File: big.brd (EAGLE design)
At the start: 77.6 x 137.2 mm, 137 parts, among them IC1 ULN2003AD, IC2 TB6612FNG, IC3 FXAS21002C, IC4 LD117ADT50TR, IC5 MCP1825, IC6 FXAS21002C, Q1 TEFT4300, Q2 TEFT4300, Q3 TEFT4300, Q4 TEFT4300, Q5 TEFT4300, Q6 TEFT4300, Q7 8MHz

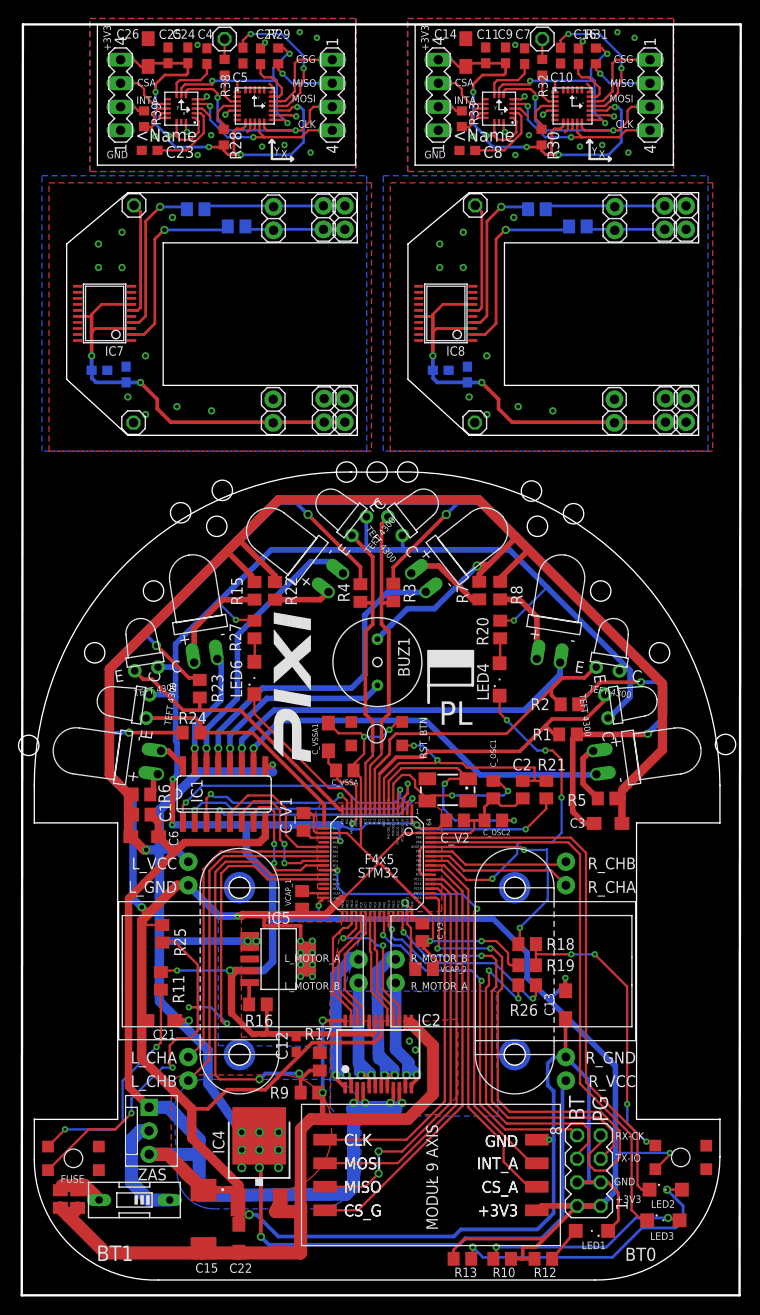
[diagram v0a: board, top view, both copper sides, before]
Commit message: schamat kodu z CubeMX
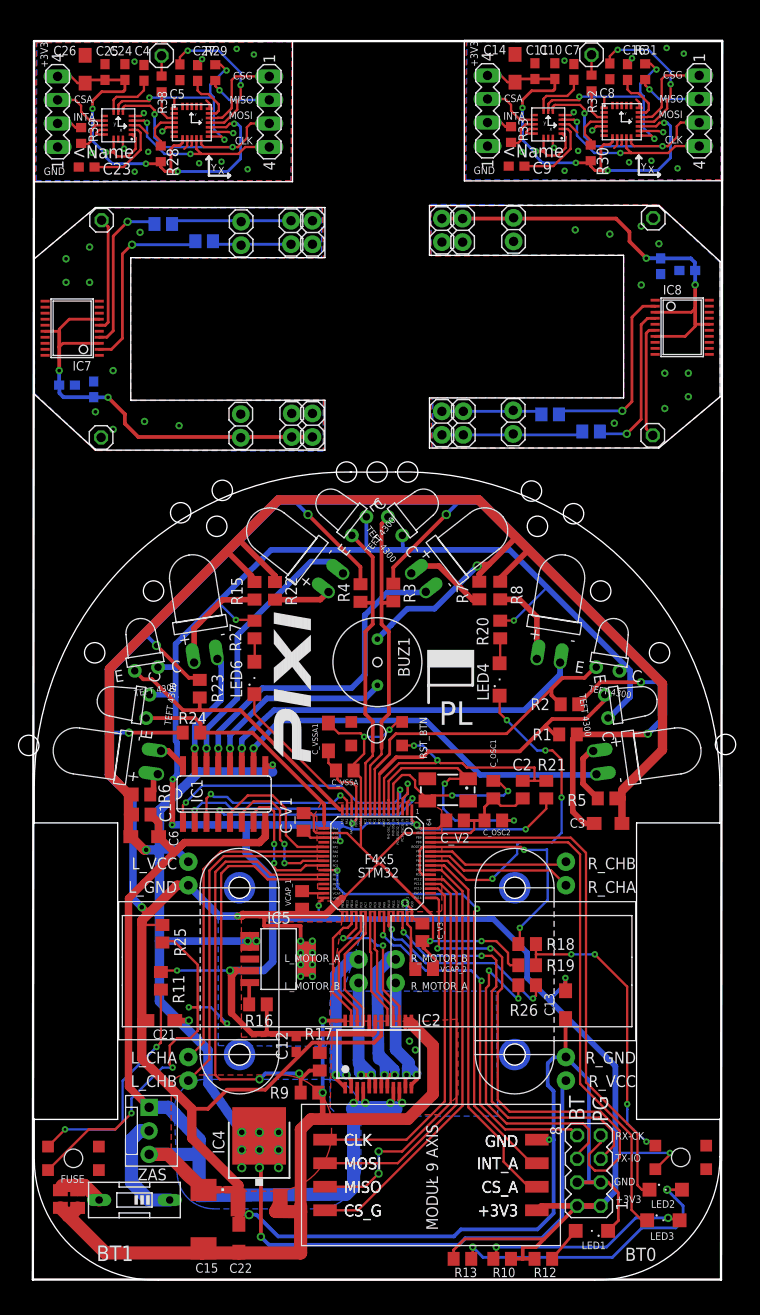
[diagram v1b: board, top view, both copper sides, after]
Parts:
- removed INT_G, JP20, JP23: (no value), pinhead:1X01
- removed JP18, JP19, JP21, JP22, JP24, JP25: PINHD_1X2_ROUND, _microMouse:PINHD_1X2_ROUND
- removed SPI: (no value), con-lstb:MA04-1
- added INT_G2, JP4, JP7: (no value), pinhead:1X01
- added JP2, JP3, JP5, JP6, JP8, JP9: PINHD_1X2_ROUND, _microMouse:PINHD_1X2_ROUND
- added SPI2: (no value), con-lstb:MA04-1
- moved C19 28.7 mm to (74.4, 109.3), turned to 0 degrees
- moved IC8 25.6 mm to (73.8, 103.2), turned to 270 degrees
- moved R37 24.7 mm to (64.0, 91.9), turned to 0 degrees
- moved C20 23.9 mm to (71.5, 109.8), turned to 270 degrees
- moved R36 20.5 mm to (59.6, 93.8), turned to 180 degrees
- moved C8 17.6 mm to (66.0, 130.8), turned to 270 degrees
- moved C9 12.0 mm to (55.9, 120.6), turned to 0 degrees
- moved SPI1 7.03 mm to (29.3, 126.5)
- moved C4 7.03 mm to (15.7, 130.7)
- moved C24 7.03 mm to (13.7, 130.7)
- moved C25 7.03 mm to (11.5, 130.7)
- moved C26 7.03 mm to (9.38, 131.1)
- moved INT_G1 7.03 mm to (17.6, 132.5)
- moved R29 7.03 mm to (23.4, 130.7)
- moved R38 7.03 mm to (17.6, 129.5)
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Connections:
- net VDDIO renamed VDDIO2
- removed net GND2: C10.2, C11.1, C14.-, C16.1, C7.2, C8.1, C9.2, IC6.GND1, IC6.GND2, IC6.GND3, IC6.GND4, IC6.RGND, IC6.RGND1, IC6.RGND2, IC6.RGND3, IC6.RGND4, IC6.RGND5, IC6.RGND6, IC6.RGND7, IC6.RGND8, U$2.P$12, U$2.P$13, U$2.P$16, U$2.P$3, U$2.P$5, ZAS1.1
- new net GND5: C10.2, C11.1, C14.-, C16.1, C7.2, C8.2, C9.1, IC6.GND1, IC6.GND2, IC6.GND3, IC6.GND4, IC6.RGND, IC6.RGND1, IC6.RGND2, IC6.RGND3, IC6.RGND4, IC6.RGND5, IC6.RGND6, IC6.RGND7, IC6.RGND8, U$2.P$12, U$2.P$13, U$2.P$16, U$2.P$3, U$2.P$5, ZAS1.1
- net +3V1: now also C10.1; no longer C9.1
- net AO2: now also JP4.1; no longer JP20.1
- net CS_G1: now also SPI2.1; no longer SPI.1
- net GND4: now also JP2.2, JP5.2, JP7.1, JP9.2; no longer JP18.2, JP21.2, JP23.1, JP25.2
- net MOSI1: now also SPI2.3; no longer SPI.3
- net N$30: now also C9.2; no longer C8.2
- net N$32: now also C8.1; no longer C10.1
- net N$36: now also SPI2.2; no longer SPI.2
- net N$37: now also INT_G2.1; no longer INT_G.1
- net N$42: now also JP3.1; no longer JP19.1
- net N$43: now also JP3.2; no longer JP19.2
- net SCLK1: now also SPI2.4; no longer SPI.4
- net VCC2: now also JP2.1; no longer JP18.1
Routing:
- net GND5: track 0.00 -> 14.8 mm, vias 0 -> 14
- net GND2: track 14.8 -> 0.00 mm, vias 14 -> 0
- added copper zone on layer 1, net GND5
- added copper zone on layer 16, net GND5
- removed copper zone on layer 1, net GND2
- removed copper zone on layer 16, net GND2
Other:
- board size 77.6 x 137.2 mm -> 74.4 x 133.8 mm
